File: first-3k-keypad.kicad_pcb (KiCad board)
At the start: 2 copper layers, 57.1 x 71.4 mm, 24 parts, among them SW1 SW_Push, U1 ATmega32U4-AU, Y1 16MHz

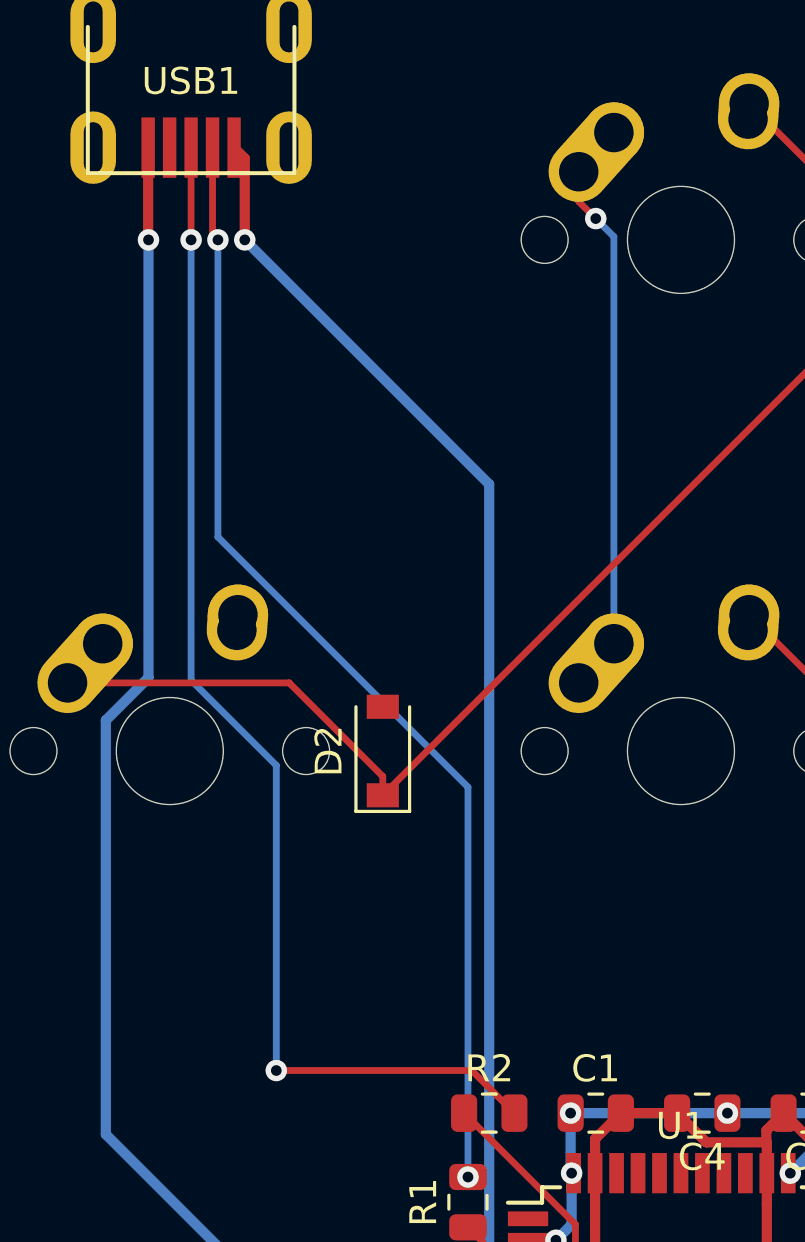
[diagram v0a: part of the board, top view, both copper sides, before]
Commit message: Minor Edits
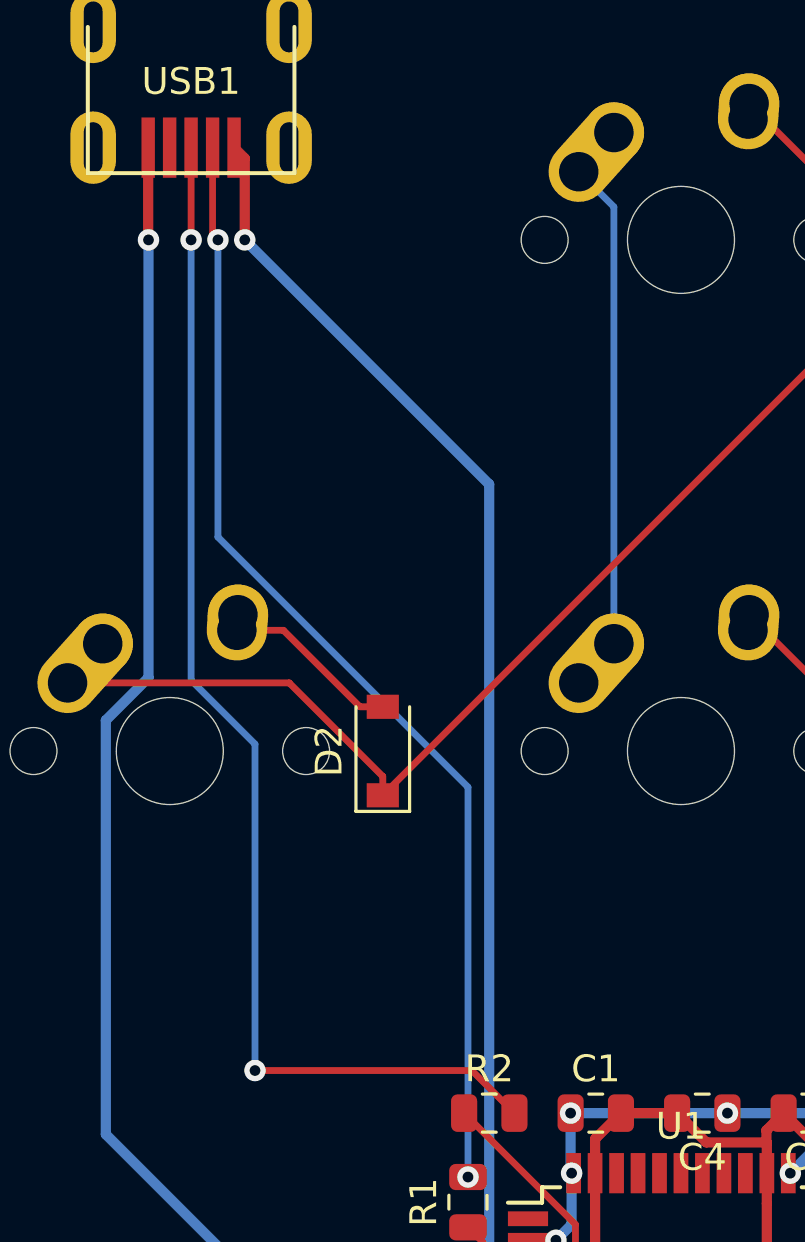
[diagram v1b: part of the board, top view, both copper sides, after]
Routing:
- net Net-(D2-Pad2): track 0.00 -> 6.62 mm
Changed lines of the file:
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@@
     (thickness 1.6)
     (drawings 9)
-    (tracks 172)
+    (tracks 173)
     (zones 0)
     (modules 24)
@@
     (0 F.Cu signal)
     (31 B.Cu signal)
-    (32 B.Adhes user)
-    (33 F.Adhes user)
-    (34 B.Paste user)
-    (35 F.Paste user)
-    (36 B.SilkS user)
-    (37 F.SilkS user)
-    (38 B.Mask user)
-    (39 F.Mask user)
-    (40 Dwgs.User user)
-    (41 Cmts.User user)
-    (42 Eco1.User user)
-    (43 Eco2.User user)
-    (44 Edge.Cuts user)
-    (45 Margin user)
-    (46 B.CrtYd user)
-    (47 F.CrtYd user)
-    (48 B.Fab user)
-    (49 F.Fab user)
+    (32 B.Adhes user hide)
+    (33 F.Adhes user hide)
+    (34 B.Paste user hide)
+    (35 F.Paste user hide)
+    (36 B.SilkS user hide)
+    (37 F.SilkS user hide)
+    (38 B.Mask user hide)
+    (39 F.Mask user hide)
+    (40 Dwgs.User user hide)
+    (41 Cmts.User user hide)
+    (42 Eco1.User user hide)
+    (43 Eco2.User user hide)
+    (44 Edge.Cuts user hide)
+    (45 Margin user hide)
+    (46 B.CrtYd user hide)
+    (47 F.CrtYd user hide)
+    (48 B.Fab user hide)
+    (49 F.Fab user hide)
   )
   (setup
@@
   (segment (start 132.97 103.125) (end 129.54 99.695) (width 0.254) (layer F.Cu) (net 6))
   (segment (start 134.9375 103.125) (end 132.97 103.125) (width 0.254) (layer F.Cu) (net 6))
+  (segment (start 115.0335 122.175) (end 115.8875 122.175) (width 0.254) (layer F.Cu) (net 7))
+  (segment (start 112.1835 119.325) (end 115.0335 122.175) (width 0.254) (layer F.Cu) (net 7))
+  (segment (start 110.45 119.325) (end 112.1835 119.325) (width 0.254) (layer F.Cu) (net 7))
   (segment (start 130.12 119.325) (end 129.5 119.325) (width 0.254) (layer F.Cu) (net 9))
   (segment (start 132.97 122.175) (end 130.12 119.325) (width 0.254) (layer F.Cu) (net 9))
@@
   (segment (start 119.853001 113.884245) (end 119.853001 146.659499) (width 0.381) (layer B.Cu) (net 10))
   (segment (start 110.743756 104.775) (end 119.853001 113.884245) (width 0.381) (layer B.Cu) (net 10))
-  (via (at 123.825 103.98125) (size 0.8) (drill 0.4) (layers F.Cu B.Cu) (net 11))
-  (segment (start 123.19 102.235) (end 123.19 103.34625) (width 0.254) (layer F.Cu) (net 11))
-  (segment (start 123.19 103.34625) (end 123.825 103.98125) (width 0.254) (layer F.Cu) (net 11))
   (via (at 124.5 119.825) (size 0.8) (drill 0.4) (layers F.Cu B.Cu) (net 11))
-  (segment (start 123.825 103.98125) (end 124.5 104.65625) (width 0.254) (layer B.Cu) (net 11))
-  (segment (start 124.5 104.65625) (end 124.5 119.825) (width 0.254) (layer B.Cu) (net 11))
+  (segment (start 124.5 103.545) (end 123.19 102.235) (width 0.254) (layer B.Cu) (net 11))
+  (segment (start 124.5 119.825) (end 124.5 103.545) (width 0.254) (layer B.Cu) (net 11))
+  (via (at 123.19 102.235) (size 0.8) (drill 0.4) (layers F.Cu B.Cu) (net 11))
   (segment (start 115.8875 124.771) (end 115.8875 125.475) (width 0.254) (layer F.Cu) (net 12))
   (segment (start 112.4015 121.285) (end 115.8875 124.771) (width 0.254) (layer F.Cu) (net 12))
@@
   (via (at 108.74375 104.775) (size 0.8) (drill 0.4) (layers F.Cu B.Cu) (net 15))
   (segment (start 108.74375 101.3375) (end 108.74375 104.775) (width 0.254) (layer F.Cu) (net 15))
-  (via (at 111.91875 135.73125) (size 0.8) (drill 0.4) (layers F.Cu B.Cu) (net 15))
-  (segment (start 111.91875 124.358816) (end 111.91875 135.73125) (width 0.254) (layer B.Cu) (net 15))
   (segment (start 108.74375 104.775) (end 108.74375 121.183816) (width 0.254) (layer B.Cu) (net 15))
-  (segment (start 108.74375 121.183816) (end 111.91875 124.358816) (width 0.254) (layer B.Cu) (net 15))
   (segment (start 119.20625 135.73125) (end 120.79375 137.31875) (width 0.254) (layer F.Cu) (net 15))
-  (segment (start 111.91875 135.73125) (end 119.20625 135.73125) (width 0.254) (layer F.Cu) (net 15))
+  (via (at 111.125 135.73125) (size 0.8) (drill 0.4) (layers F.Cu B.Cu) (net 15))
+  (segment (start 108.74375 121.183816) (end 111.125 123.565066) (width 0.254) (layer B.Cu) (net 15))
+  (segment (start 111.125 123.565066) (end 111.125 135.73125) (width 0.254) (layer B.Cu) (net 15))
+  (segment (start 111.125 135.73125) (end 119.20625 135.73125) (width 0.254) (layer F.Cu) (net 15))
   (segment (start 122.304 143.65625) (end 121.3 143.65625) (width 0.254) (layer F.Cu) (net 16))
   (segment (start 123.067477 142.892773) (end 122.304 143.65625) (width 0.254) (layer F.Cu) (net 16))
